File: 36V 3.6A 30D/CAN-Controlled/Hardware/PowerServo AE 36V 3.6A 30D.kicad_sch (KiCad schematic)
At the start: 26 parts, among them J1 Control_In, J2 MOT_A, J3 Prog_IN, J4 Power_In, J6 Control_In, J7 MOT_B, U1 LMZM23601V5, U2 TLV76733DRVx, U3 DRV8871DDA, U4 MA730, U5 TJA1051T-3, U7 STM32G0B1KBTx

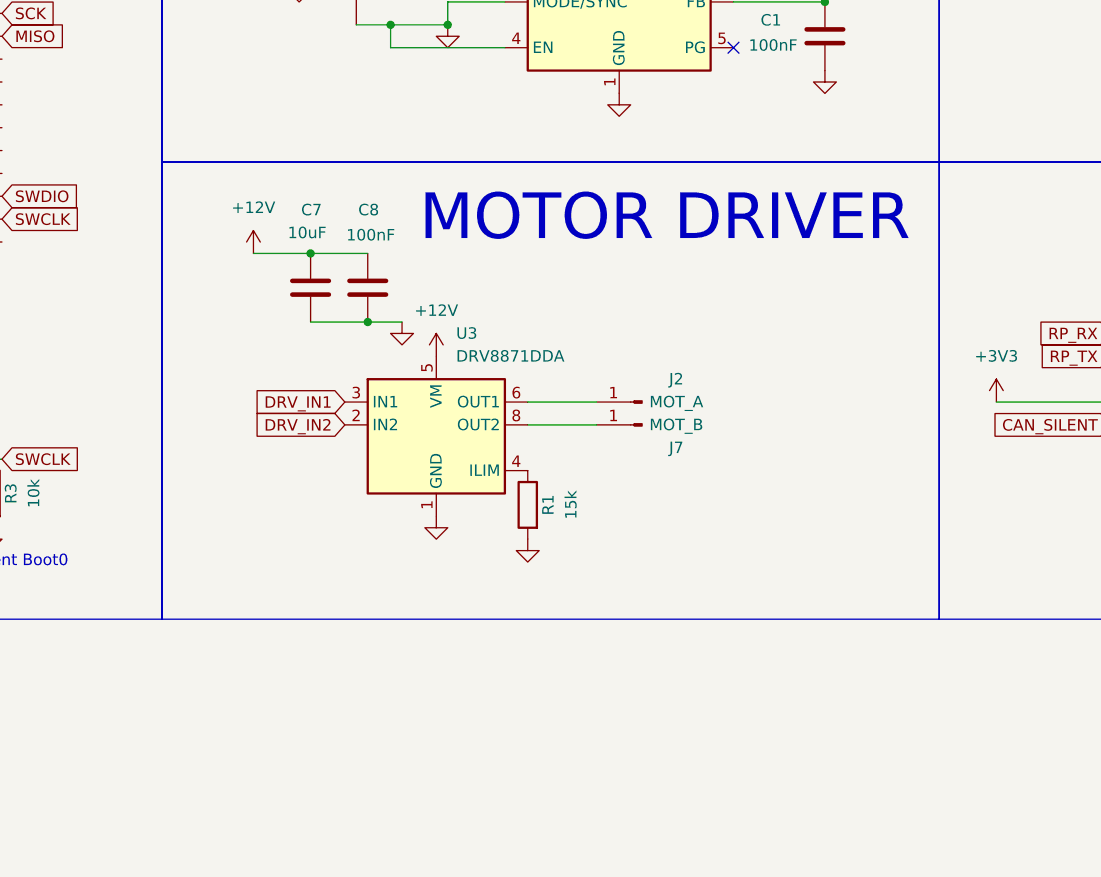
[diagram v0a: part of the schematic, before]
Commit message: Finalized Reddit TODO
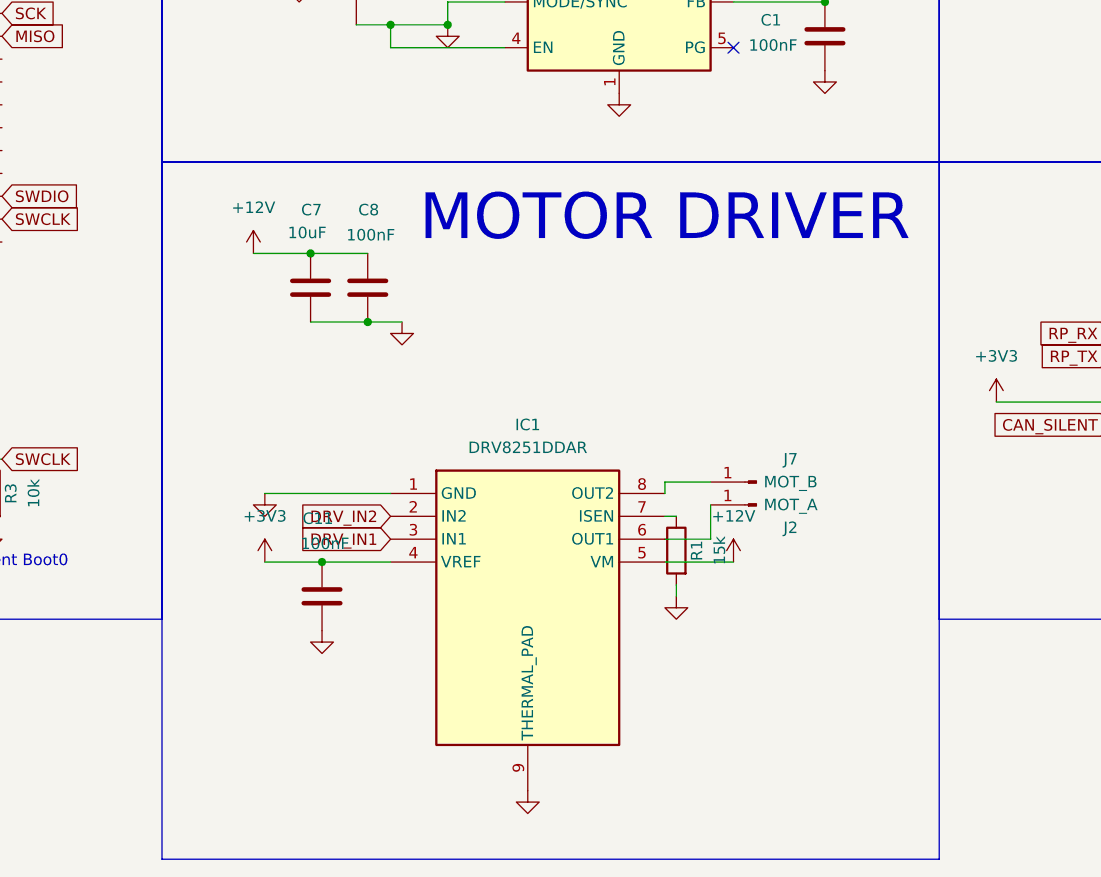
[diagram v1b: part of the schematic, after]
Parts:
- removed U3: DRV8871DDA, Package_SO:Texas_HTSOP-8-1EP_3.9x4.9mm_P1.27mm_EP2.95x4.9mm_Mask2.4x3.1mm_ThermalVias, symbol Driver_Motor:DRV8871DDA
- added C11: 100nF, Capacitor_SMD:C_0603_1608Metric, symbol Device:C
- added IC1: DRV8251DDAR, SOIC127P600X170-9N, symbol _Custom:DRV8251DDAR
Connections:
- net +12V: now also IC1.5 (VM)
- net +3V3: now also C11.2, IC1.4 (VREF)
- net DRV_IN1: now also IC1.3 (IN1)
- net DRV_IN2: now also IC1.2 (IN2)
- net GND: now also C11.1, IC1.1 (GND), IC1.9 (THERMAL_PAD)
- net at J2.1 (Pin_1): now also IC1.6 (OUT1)
- net at R1.1: now also IC1.7 (ISEN)
- net at J7.1 (Pin_1): now also IC1.8 (OUT2)
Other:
- moved on the sheet: J2, J7, R1
